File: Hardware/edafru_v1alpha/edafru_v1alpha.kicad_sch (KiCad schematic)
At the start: 0 parts

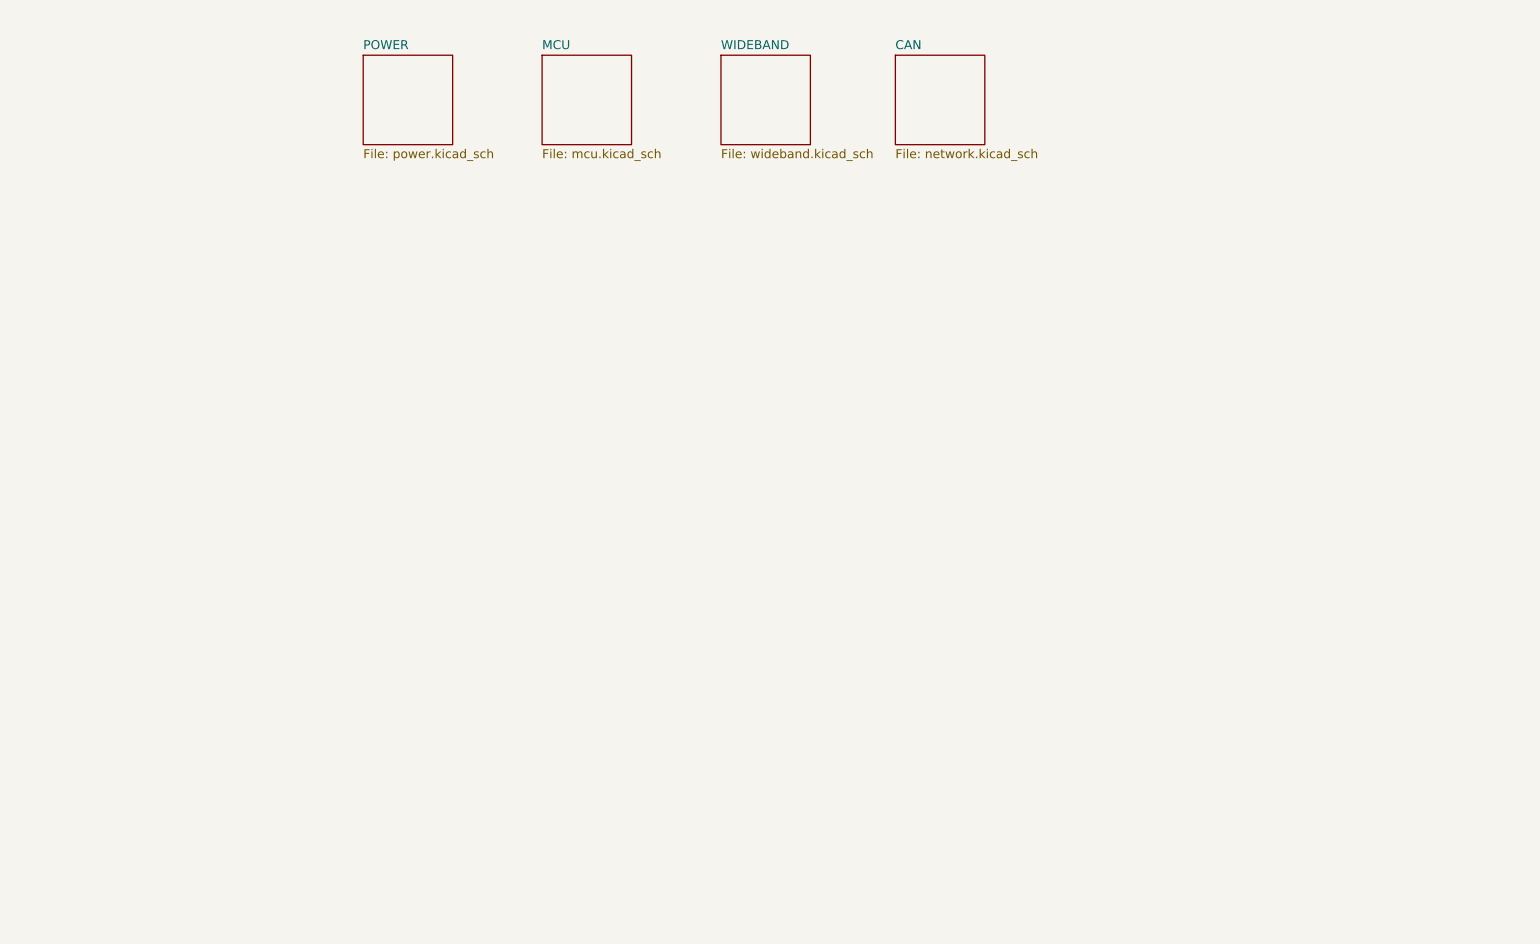
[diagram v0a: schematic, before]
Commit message: PCB is developing...
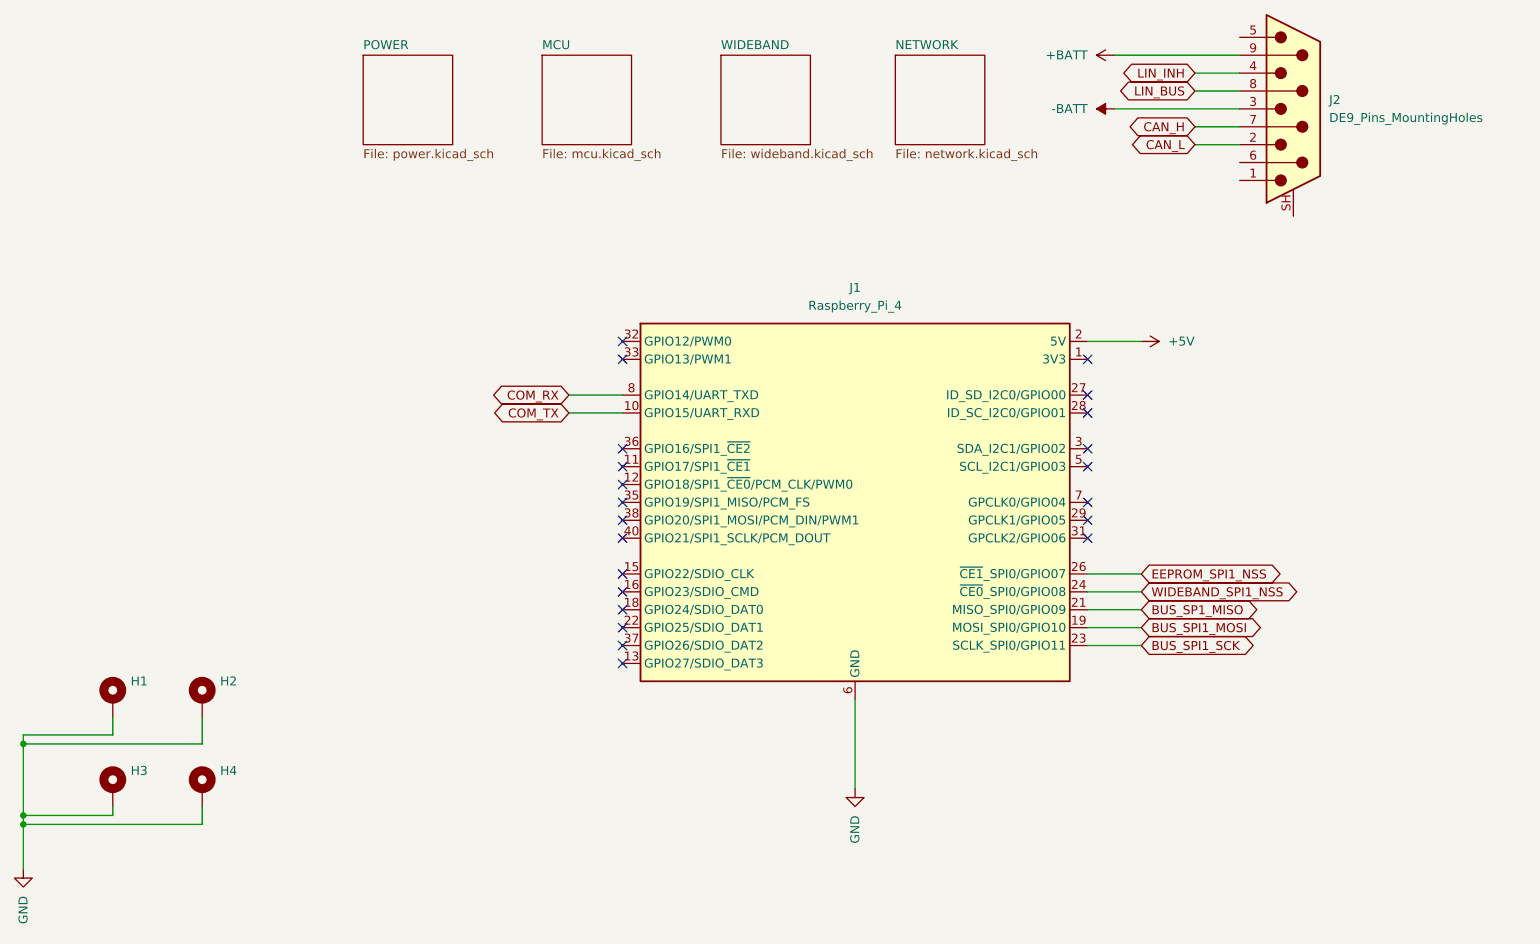
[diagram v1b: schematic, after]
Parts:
- added H1, H2, H3, H4: MountingHole_Pad_MP, MountingHole:MountingHole_3.2mm_M3_ISO14580_Pad, symbol Mechanical:MountingHole_Pad_MP
- added J1: Raspberry_Pi_4, Connector_PinSocket_2.54mm:PinSocket_2x20_P2.54mm_Vertical, symbol Connector:Raspberry_Pi_4
- added J2: DE9_Pins_MountingHoles, Connector_Dsub:DSUB-9_Pins_Horizontal_P2.77x2.84mm_EdgePinOffset4.94mm_Housed_MountingHolesOffset4.94mm, symbol Connector:DE9_Pins_MountingHoles
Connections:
- new net: J1.1 (3V3), J1.17 (3V3)
- new net +5V: J1.2 (5V), J1.4 (5V)
- new net +BATT: J2.9
- new net -BATT: J2.3
- new net BUS_SP1_MISO: J1.21 (MISO_SPI0/GPIO09)
- new net BUS_SPI1_MOSI: J1.19 (MOSI_SPI0/GPIO10)
- new net BUS_SPI1_SCK: J1.23 (SCLK_SPI0/GPIO11)
- new net CAN_H: J2.7
- new net CAN_L: J2.2
- new net COM_RX: J1.8 (GPIO14/UART_TXD)
- new net COM_TX: J1.10 (GPIO15/UART_RXD)
- new net EEPROM_SPI1_NSS: J1.26 (~{CE1}_SPI0/GPIO07)
- new net GND: H1.MP, H2.MP, H3.MP, H4.MP, J1.14 (GND), J1.20 (GND), J1.25 (GND), J1.30 (GND), J1.34 (GND), J1.39 (GND), J1.6 (GND), J1.9 (GND)
- new net LIN_BUS: J2.8
- new net LIN_INH: J2.4
- new net WIDEBAND_SPI1_NSS: J1.24 (~{CE0}_SPI0/GPIO08)
- no-connect marks 0 -> 22
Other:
- sheet CAN renamed NETWORK
